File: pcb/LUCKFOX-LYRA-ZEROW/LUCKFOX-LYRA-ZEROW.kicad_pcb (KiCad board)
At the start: 2 copper layers, 3 parts, among them U1 Luckfox_Lyra_Zero_W, U2 ME54BS12-nRF54L15, U3 ME54BS01-nRF54L15

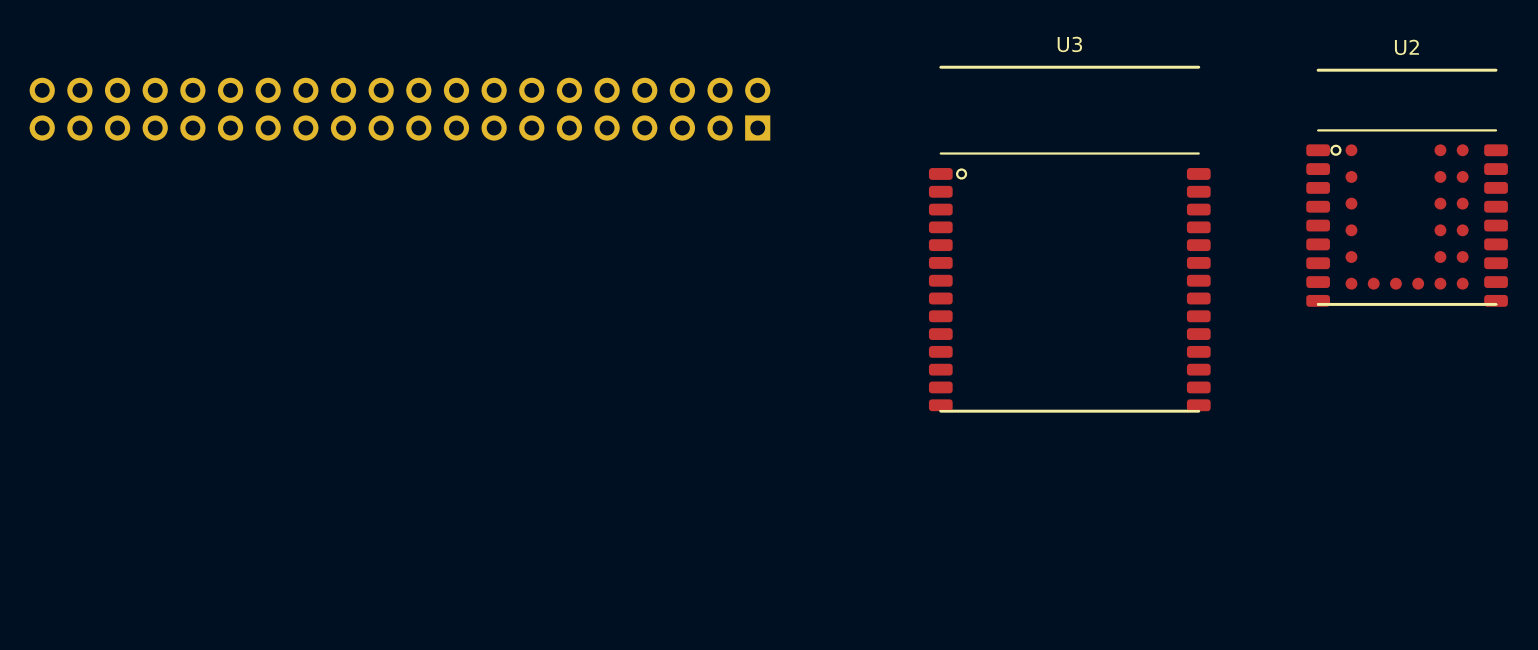
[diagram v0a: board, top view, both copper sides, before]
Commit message: more pcb work
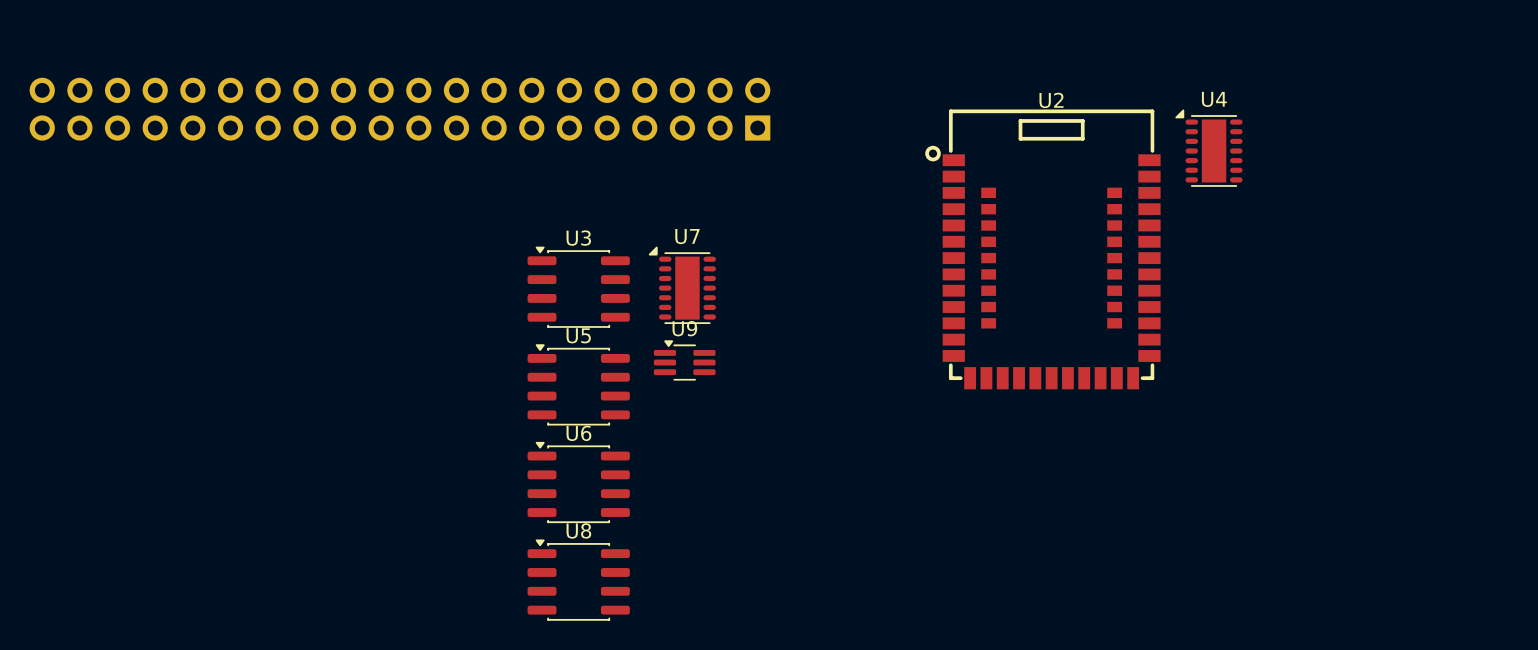
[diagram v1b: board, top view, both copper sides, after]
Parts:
- added U4: MCP2518FD-xQBB, Package_DFN_QFN:DFN-14-1EP_3x4.5mm_P0.65mm_EP1.65x4.25mm, F.Cu at (132.7, 46.8)
- added U5: MAX3051, Package_SO:SOIC-8_3.9x4.9mm_P1.27mm, F.Cu at (89.9, 62.7)
- added U6: MAX3051, Package_SO:SOIC-8_3.9x4.9mm_P1.27mm, F.Cu at (89.9, 69.3)
- added U7: MCP2518FD-xQBB, Package_DFN_QFN:DFN-14-1EP_3x4.5mm_P0.65mm_EP1.65x4.25mm, F.Cu at (97.2, 56.0)
- added U8: MAX3051, Package_SO:SOIC-8_3.9x4.9mm_P1.27mm, F.Cu at (89.9, 75.9)
- added U9: 74AUP2G34GW,125, Package_TO_SOT_SMD:SOT-363_SC-70-6_Handsoldering, F.Cu at (97.0, 61.1)
- U2: value ME54BS12-nRF54L15 -> CORE52840; footprint MinewSemi_nRF54:ME54BS12_nRF54L15 -> Core52840:BULETM-SMD_HOLYIOT-18010-NRF52840
- U3: value ME54BS01-nRF54L15 -> MAX3051; footprint MinewSemi_nRF54:ME54BS01_nRF54L15 -> Package_SO:SOIC-8_3.9x4.9mm_P1.27mm
- moved U3 33.3 mm to (89.9, 56.1)
- moved U2 24.6 mm to (121.8, 54.8)
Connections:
- U1 pad 1: unconnected-(U1-3V3-Pad1) -> +3.3VA
- U1 pad 14: unconnected-(U1-GND-Pad14) -> GND
- U1 pad 17: unconnected-(U1-3V3-Pad17) -> +3.3VA
- U1 pad 2: unconnected-(U1-5V-Pad2) -> +5V
- U1 pad 20: unconnected-(U1-GND-Pad20) -> GND
- U1 pad 25: unconnected-(U1-GND-Pad25) -> GND
- U1 pad 30: unconnected-(U1-GND-Pad30) -> GND
- U1 pad 34: unconnected-(U1-GND-Pad34) -> GND
- U1 pad 39: unconnected-(U1-GND-Pad39) -> GND
- U1 pad 4: unconnected-(U1-5V-Pad4) -> +5V
- U1 pad 6: unconnected-(U1-GND-Pad6) -> GND
- U1 pad 9: unconnected-(U1-GND-Pad9) -> GND
- U2 pad 1: unconnected-(U2-RF-Pad1) -> GND
- U2 pad 14: unconnected-(U2-P0.02-Pad14) -> +3V3
- U3 pad 2: unconnected-(U3-P1.09-Pad2) -> GND
- U3 pad 3: unconnected-(U3-P1.10-Pad3) -> +3.3VA
- U3 pad 8: unconnected-(U3-P1.06-Pad8) -> GND
